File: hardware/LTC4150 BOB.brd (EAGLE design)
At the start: 15.2 x 30.5 mm, 23 parts, among them U1 LTC4150

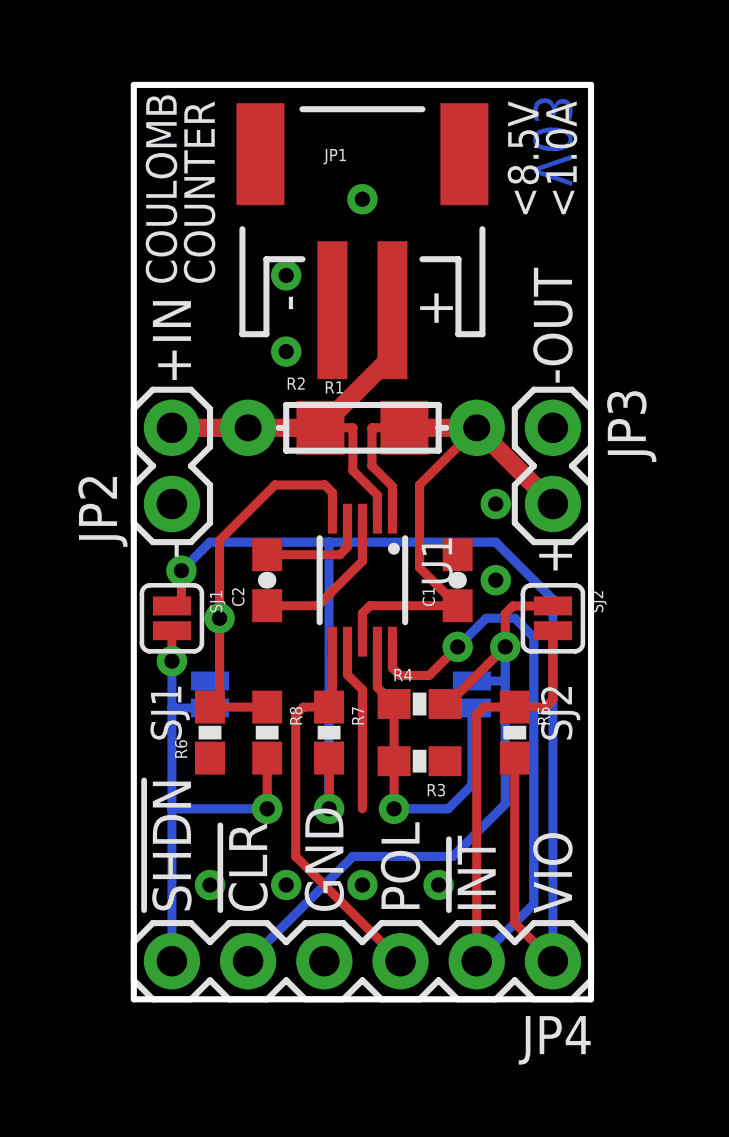
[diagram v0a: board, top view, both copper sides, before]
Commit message: Changed temp parts to SparkFun library variants
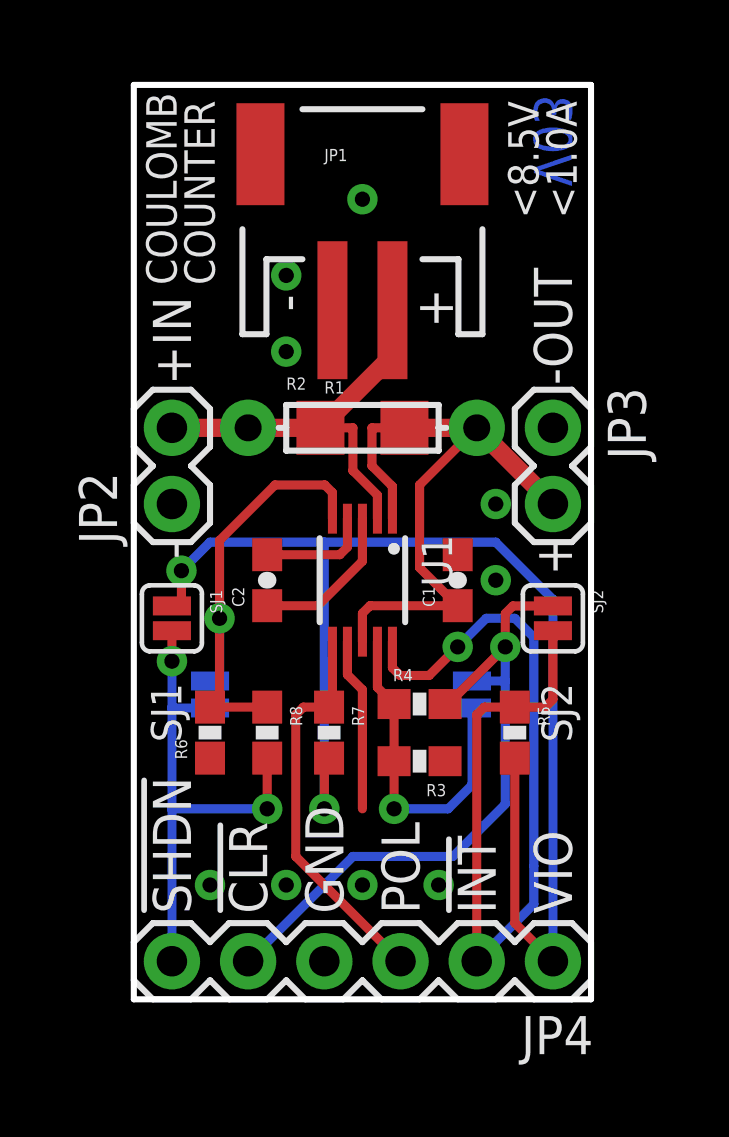
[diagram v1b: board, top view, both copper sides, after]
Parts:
- SJ1: device mike-temp:SJ_2S -> SparkFun-Passives:SJ_2S
- SJ3, SJ4: device mike-temp:SJ_2S-NO -> SparkFun-Passives:SJ_2S-NO
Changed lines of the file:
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@@
 <?xml version="1.0" encoding="utf-8"?>
 <!DOCTYPE eagle SYSTEM "eagle.dtd">
-<eagle version="6.4">
+<eagle version="6.5.0">
 <drawing>
 <settings>
@@
 <grid distance="0.05" unitdist="inch" unit="inch" style="lines" multiple="2" display="yes" altdistance="0.00625" altunitdist="inch" altunit="inch"/>
 <layers>
-<layer number="1" name="Top" color="4" fill="1" visible="no" active="yes"/>
+<layer number="1" name="Top" color="4" fill="1" visible="yes" active="yes"/>
 <layer number="2" name="Route2" color="1" fill="3" visible="no" active="no"/>
 <layer number="3" name="Route3" color="4" fill="3" visible="no" active="no"/>
@@
 <layer number="14" name="Route14" color="1" fill="6" visible="no" active="no"/>
 <layer number="15" name="Route15" color="4" fill="6" visible="no" active="no"/>
-<layer number="16" name="Bottom" color="1" fill="1" visible="yes" active="yes"/>
+<layer number="16" name="Bottom" color="1" fill="1" visible="no" active="yes"/>
 <layer number="17" name="Pads" color="2" fill="1" visible="yes" active="yes"/>
 <layer number="18" name="Vias" color="2" fill="1" visible="yes" active="yes"/>
 <layer number="19" name="Unrouted" color="6" fill="1" visible="yes" active="yes"/>
 <layer number="20" name="Dimension" color="15" fill="1" visible="yes" active="yes"/>
-<layer number="21" name="tPlace" color="7" fill="1" visible="no" active="yes"/>
-<layer number="22" name="bPlace" color="7" fill="1" visible="yes" active="yes"/>
-<layer number="23" name="tOrigins" color="15" fill="1" visible="no" active="yes"/>
+<layer number="21" name="tPlace" color="7" fill="1" visible="yes" active="yes"/>
+<layer number="22" name="bPlace" color="7" fill="1" visible="no" active="yes"/>
+<layer number="23" name="tOrigins" color="15" fill="1" visible="yes" active="yes"/>
 <layer number="24" name="bOrigins" color="15" fill="1" visible="no" active="yes"/>
 <layer number="25" name="tNames" color="7" fill="1" visible="no" active="yes"/>
@@
 <layer number="27" name="tValues" color="7" fill="1" visible="no" active="yes"/>
 <layer number="28" name="bValues" color="7" fill="1" visible="no" active="yes"/>
-<layer number="29" name="tStop" color="7" fill="3" visible="no" active="yes"/>
+<layer number="29" name="tStop" color="7" fill="3" visible="yes" active="yes"/>
 <layer number="30" name="bStop" color="7" fill="6" visible="no" active="yes"/>
-<layer number="31" name="tCream" color="7" fill="4" visible="no" active="yes"/>
+<layer number="31" name="tCream" color="7" fill="4" visible="yes" active="yes"/>
 <layer number="32" name="bCream" color="7" fill="5" visible="no" active="yes"/>
 <layer number="33" name="tFinish" color="6" fill="3" visible="no" active="yes"/>
@@
 <layer number="49" name="Reference" color="7" fill="1" visible="no" active="yes"/>
 <layer number="50" name="dxf" color="7" fill="1" visible="no" active="no"/>
-<layer number="51" name="tDocu" color="7" fill="1" visible="no" active="yes"/>
+<layer number="51" name="tDocu" color="7" fill="1" visible="yes" active="yes"/>
 <layer number="52" name="bDocu" color="7" fill="1" visible="no" active="yes"/>
 <layer number="53" name="tGND_GNDA" color="7" fill="9" visible="no" active="no"/>
@@
 <dimension x1="0" y1="0" x2="0" y2="30.48" x3="-2.54" y3="15.24" textsize="1.27" textratio="15" layer="51" unit="inch" precision="1"/>
 <dimension x1="0" y1="30.48" x2="15.24" y2="30.48" x3="7.62" y3="33.02" textsize="1.27" textratio="15" layer="51" unit="inch" precision="1"/>
-<text x="8.89" y="-11.43" size="1.778" layer="27">M Grusin</text>
+<text x="8.89" y="-11.43" size="1.778" layer="51">M Grusin</text>
 <text x="13.49375" y="26.035" size="1.016" layer="21" ratio="15" rot="R90">&lt;8.5V</text>
 <text x="14.76375" y="26.035" size="1.016" layer="21" ratio="15" rot="R90">&lt;1.0A</text>
@@
 <element name="LOGO3" library="SparkFun-Aesthetics" package="SFE-LOGO-FLAME" value="LOGO-SFESK" x="8.89" y="26.67" rot="MR90"/>
 <element name="LOGO1" library="SparkFun-Aesthetics" package="OSHW-LOGO-S" value="OSHW-LOGOS" x="1.905" y="28.2575" rot="MR90"/>
-<element name="SJ3" library="mike-temp" package="SJ_2S-NO" value="" x="11.27125" y="10.16" rot="MR90"/>
-<element name="SJ1" library="mike-temp" package="SJ_2S" value="" x="1.27" y="12.7" rot="R270"/>
+<element name="SJ3" library="SparkFun-Passives" package="SJ_2S-NO" value="" x="11.27125" y="10.16" rot="MR90"/>
+<element name="SJ1" library="SparkFun-Passives" package="SJ_2S" value="" x="1.27" y="12.7" rot="R270"/>
 <element name="LOGO2" library="SparkFun-Aesthetics" package="SFE-NEW-WEB" value="LOGO-SFENW2" x="8.255" y="13.97" rot="MR90"/>
 <element name="SJ2" library="SparkFun-Passives" package="SJ_2S" value="" x="13.97" y="12.7" rot="R270"/>
@@
 <attribute name="NAME" x="5.08" y="20.32" size="0.4064" layer="25" font="vector"/>
 </element>
-<element name="SJ4" library="mike-temp" package="SJ_2S-NO" value="" x="2.54" y="10.16" rot="MR270"/>
+<element name="SJ4" library="SparkFun-Passives" package="SJ_2S-NO" value="" x="2.54" y="10.16" rot="MR270"/>
 </elements>
 <signals>
@@
 <contactref element="JP4" pad="1"/>
 <wire x1="12.7" y1="8.04" x2="12.7" y2="2.54" width="0.3048" layer="1"/>
-<wire x1="6.50875" y1="8.04" x2="6.50875" y2="6.35" width="0.3048" layer="1"/>
-<via x="6.50875" y="6.35" extent="1-16" drill="0.508"/>
+<wire x1="6.50875" y1="8.04" x2="6.35" y2="8.04" width="0.3048" layer="1"/>
+<wire x1="6.35" y1="8.04" x2="6.35" y2="7.9375" width="0.3048" layer="1"/>
+<wire x1="6.35" y1="7.9375" x2="6.35" y2="6.35" width="0.3048" layer="1"/>
+<via x="6.35" y="6.35" extent="1-16" drill="0.508"/>
 <wire x1="12.7" y1="2.54" x2="13.97" y2="1.27" width="0.3048" layer="1"/>
 <contactref element="SJ1" pad="1"/>
-<wire x1="6.50875" y1="6.35" x2="6.50875" y2="15.24" width="0.3048" layer="16"/>
-<wire x1="6.50875" y1="15.24" x2="12.065" y2="15.24" width="0.3048" layer="16"/>
+<wire x1="6.35" y1="6.35" x2="6.35" y2="7.62" width="0.3048" layer="16"/>
+<wire x1="6.35" y1="7.62" x2="6.35" y2="15.24" width="0.3048" layer="16"/>
+<wire x1="6.35" y1="15.24" x2="12.065" y2="15.24" width="0.3048" layer="16"/>
 <wire x1="12.065" y1="15.24" x2="13.97" y2="13.335" width="0.3048" layer="16"/>
 <wire x1="13.97" y1="13.335" x2="13.97" y2="1.27" width="0.3048" layer="16"/>
@@
 <wire x1="1.5875" y1="13.1119" x2="1.5875" y2="14.2875" width="0.3048" layer="1"/>
 <via x="1.5875" y="14.2875" extent="1-16" drill="0.508"/>
-<wire x1="6.50875" y1="15.24" x2="2.54" y2="15.24" width="0.3048" layer="16"/>
+<wire x1="6.35" y1="15.24" x2="2.54" y2="15.24" width="0.3048" layer="16"/>
 <wire x1="2.54" y1="15.24" x2="1.5875" y2="14.2875" width="0.3048" layer="16"/>
 </signal>
